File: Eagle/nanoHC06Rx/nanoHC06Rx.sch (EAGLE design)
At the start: 40 parts, among them J10 Relay, J14 Relay, J17 Relay, J2 Relay, J20 Pixel, J22 IR Rx, J33 Relay, Q1 2N5088, Q2 2N5088, X1 53047-11

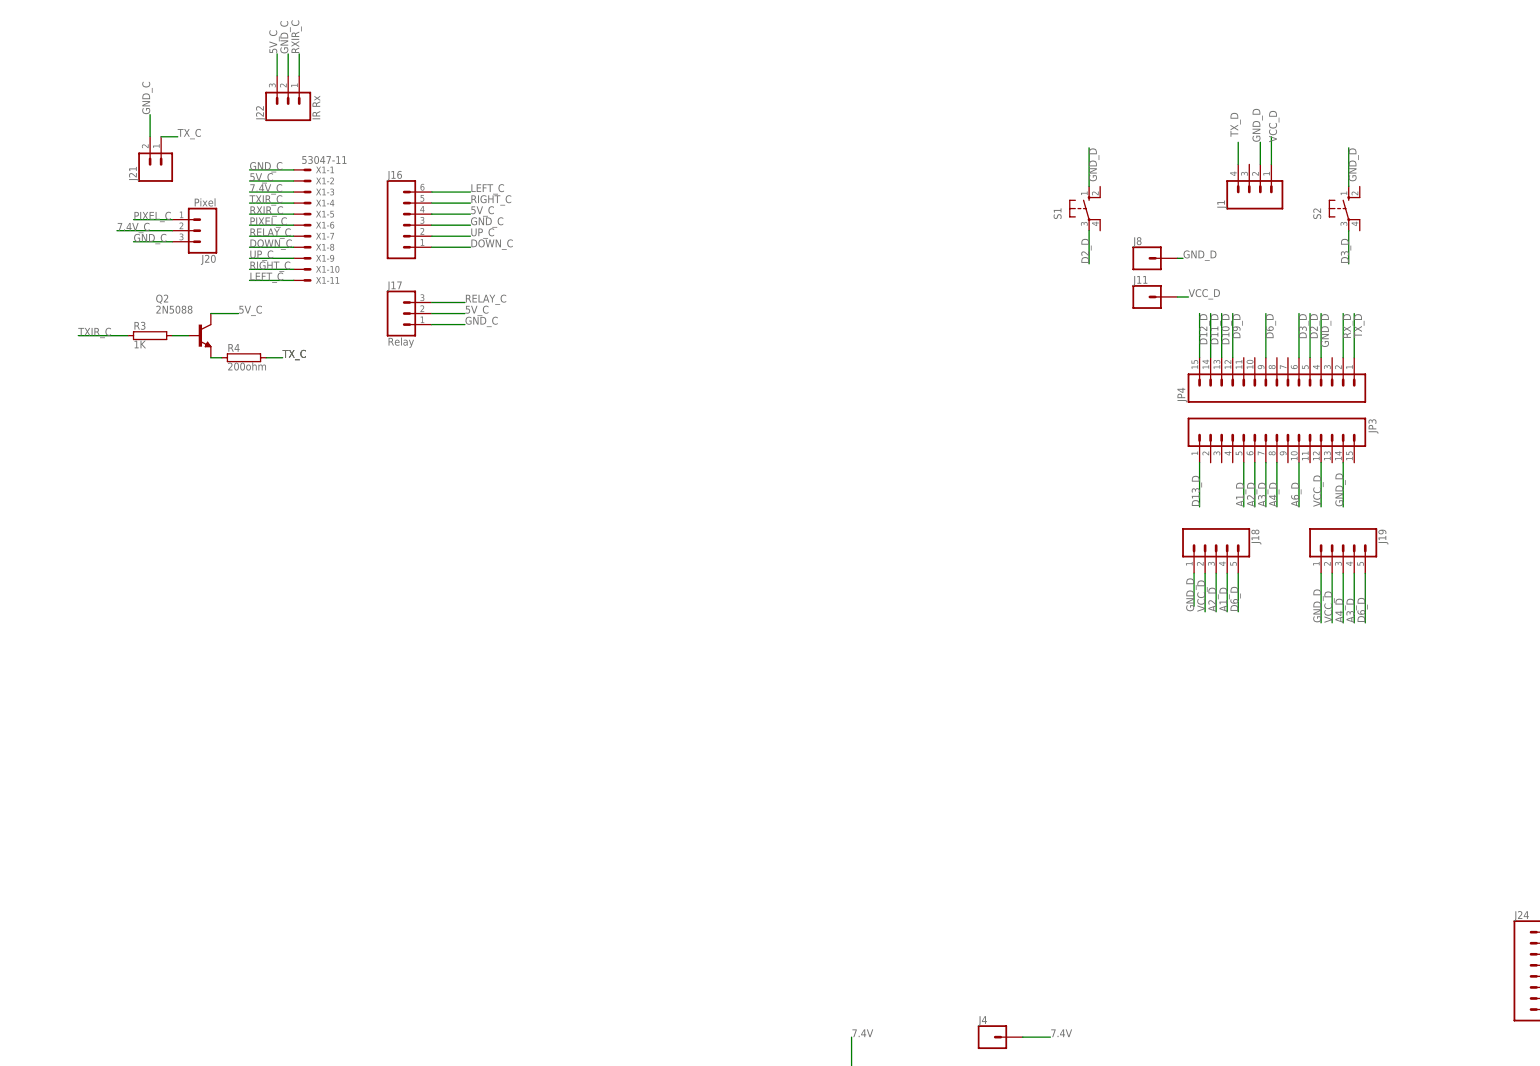
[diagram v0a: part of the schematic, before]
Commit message: eagle
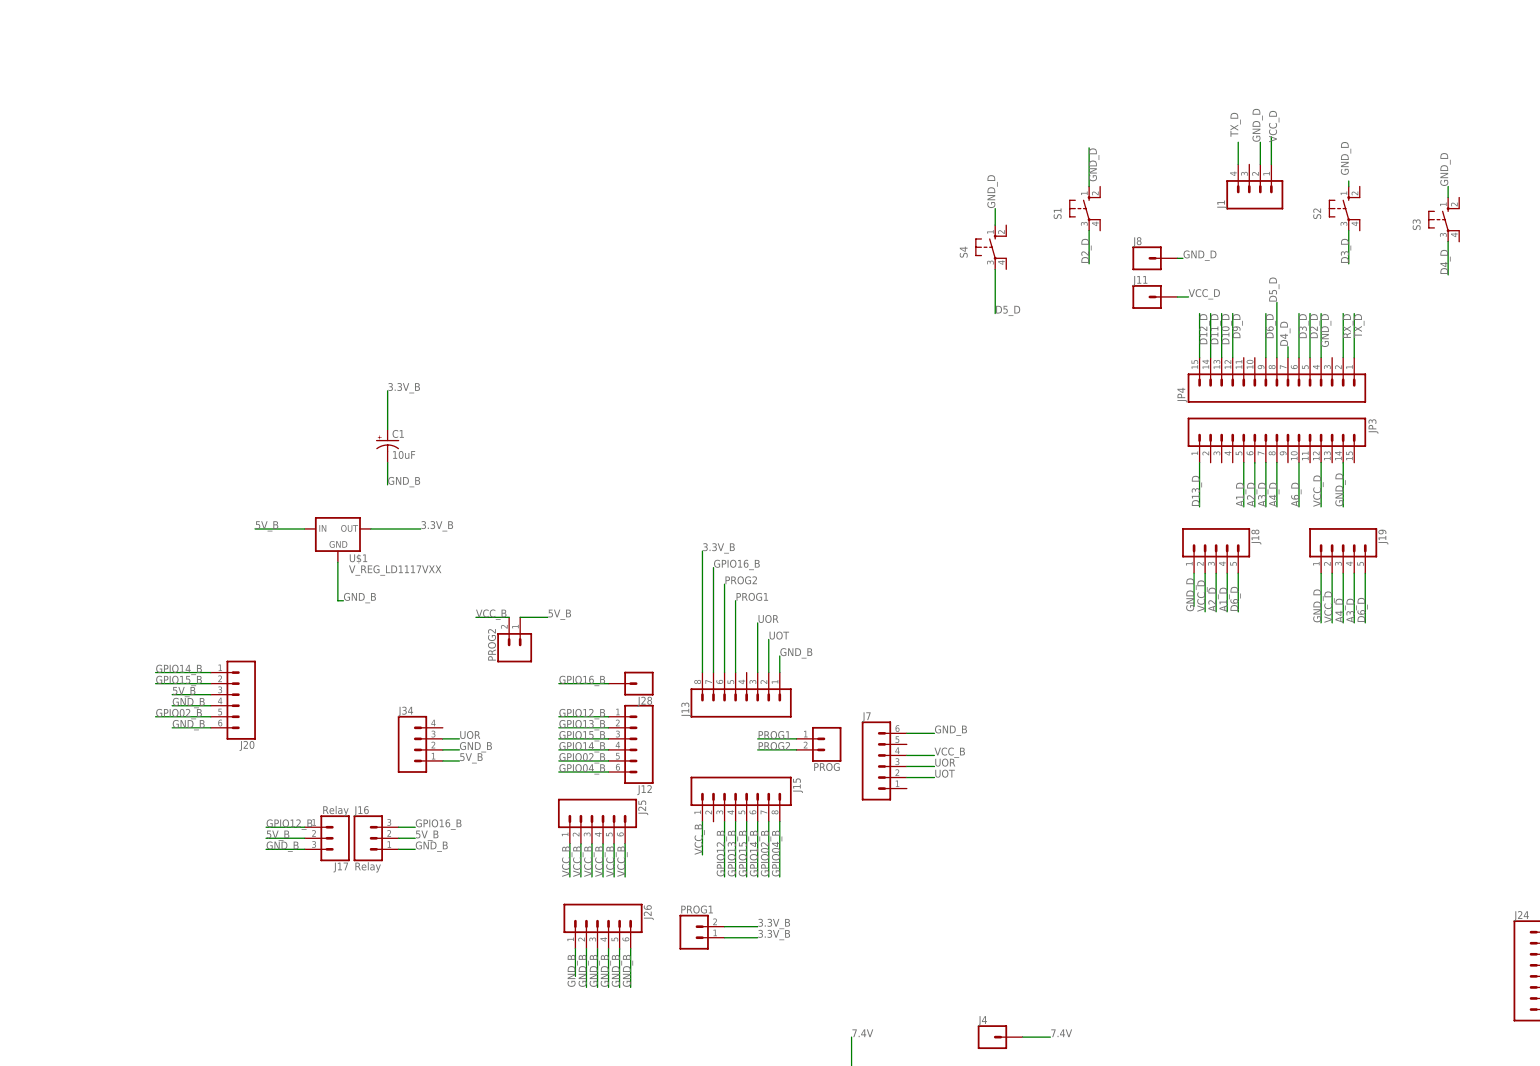
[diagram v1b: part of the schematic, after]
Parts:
- removed J21: (no value), SparkFun-Connectors:CONN_02
- removed J22: IR Rx, SparkFun-Connectors:CONN_03
- removed Q2: 2N5088, transistor-npn:2N5088
- removed R3: 1K, resistor-power:RCA0001
- removed R4: 200ohm, resistor-power:RCA0001
- removed X1: 53047-11, con-molex:53047-11
- added C1: 10uF, SparkFun-Capacitors:10UF-POLAR-RADIAL-2.5MM-KIT-25V-20%
- added J12, J25, J26, J7: (no value), SparkFun-Connectors:CONN_06NO_SILK_FEMALE_PTH
- added J13, J15: (no value), SparkFun-Connectors:CONN_08"
- added J28: (no value), SparkFun-Connectors:CONN_01
- added J34: (no value), SparkFun-Connectors:CONN_04
- added PROG, PROG1, PROG2: (no value), SparkFun-Connectors:CONN_02
- added S3, S4: (no value), switch-omron:40-XX
- added U$1: V_REG_LD1117VXX, SparkFun-IC-Power:V_REG_LD1117VXX
- J16: value (none) -> Relay; device SparkFun-Connectors:CONN_06NO_SILK_FEMALE_PTH -> SparkFun-Connectors:CONN_03
- J20: value Pixel -> (none); device SparkFun-Connectors:CONN_03 -> SparkFun-Connectors:CONN_06NO_SILK_FEMALE_PTH
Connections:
- removed net 5V_C: J16.4, J17.2, J22.3, Q2.C, X1-2.S
- removed net 7.4V_C: J20.2, X1-3.S
- removed net DOWN_C: J16.1, X1-8.S
- removed net GND_C: J16.3, J17.1, J20.3, J21.2, J22.2, X1-1.S
- removed net LEFT_C: J16.6, X1-11.S
- removed net N$2: Q2.B, R3.2
- removed net N$4: Q2.E, R4.1
- removed net PIXEL_C: J20.1, X1-6.S
- removed net RELAY_C: J17.3, X1-7.S
- removed net RIGHT_C: J16.5, X1-10.S
- removed net RXIR_C: J22.1, X1-5.S
- removed net TXIR_C: R3.1, X1-4.S
- removed net TX_C: J21.1, R4.2
- removed net UP_C: J16.2, X1-9.S
- new net 3.3V_B: C1.+, J13.8, PROG1.1, PROG1.2, U$1.OUT
- new net 5V_B: J16.2, J17.2, J20.3, J34.1, PROG2.1, U$1.IN
- new net D4_D: JP4.7, S3.P
- new net D5_D: JP4.8, S4.P
- new net GND_B: C1.-, J13.1, J16.1, J17.3, J20.4, J20.6, J26.1, J26.2, J26.3, J26.4, J26.5, J26.6, J34.2, J7.6, U$1.GND
- new net GPIO02_B: J12.5, J15.7, J20.5
- new net GPIO04_B: J12.6, J15.8
- new net GPIO12_B: J12.1, J15.3, J17.1
- new net GPIO13_B: J12.2, J15.4
- new net GPIO14_B: J12.4, J15.6, J20.1
- new net GPIO15_B: J12.3, J15.5, J20.2
- new net GPIO16_B: J13.7, J16.3, J28.1
- new net PROG1: J13.5, PROG.1
- new net PROG2: J13.6, PROG.2
- new net UOR: J13.3, J34.3, J7.3
- new net UOT: J13.2, J7.2
- new net VCC_B: J15.1, J25.1, J25.2, J25.3, J25.4, J25.5, J25.6, J7.4, PROG2.2
- net GND_D: now also S3.S, S4.S
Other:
- moved on the sheet: J17
